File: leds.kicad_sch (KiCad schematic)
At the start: 6 parts, among them IC1 HT16K33

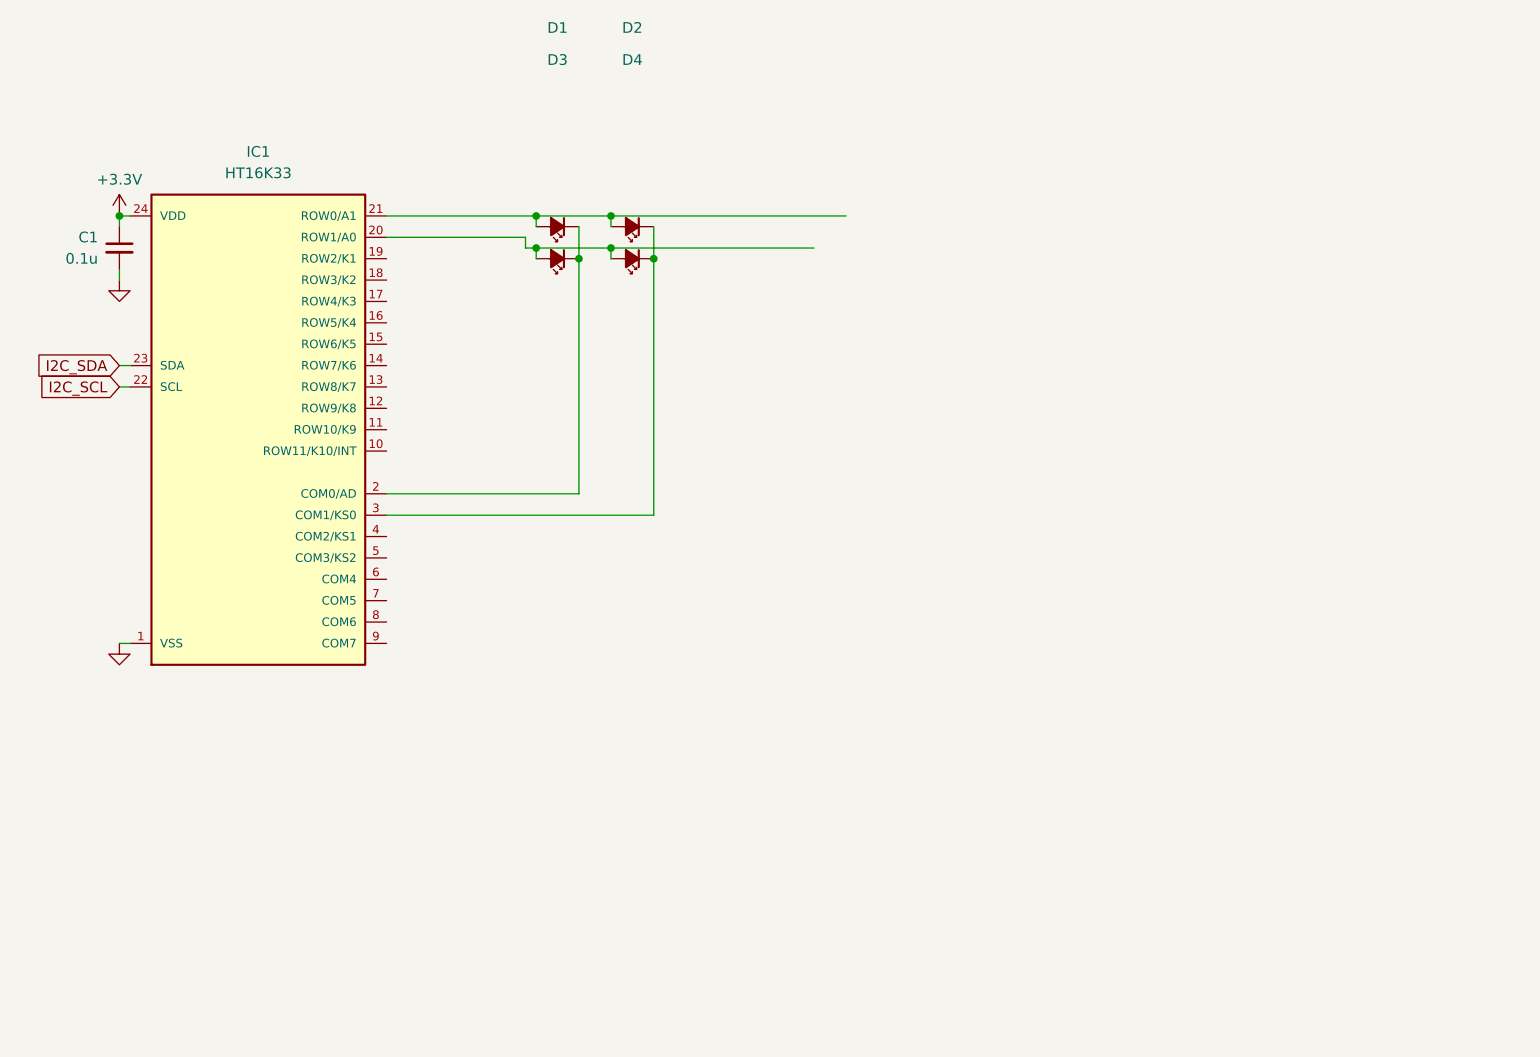
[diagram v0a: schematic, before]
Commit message: 251023
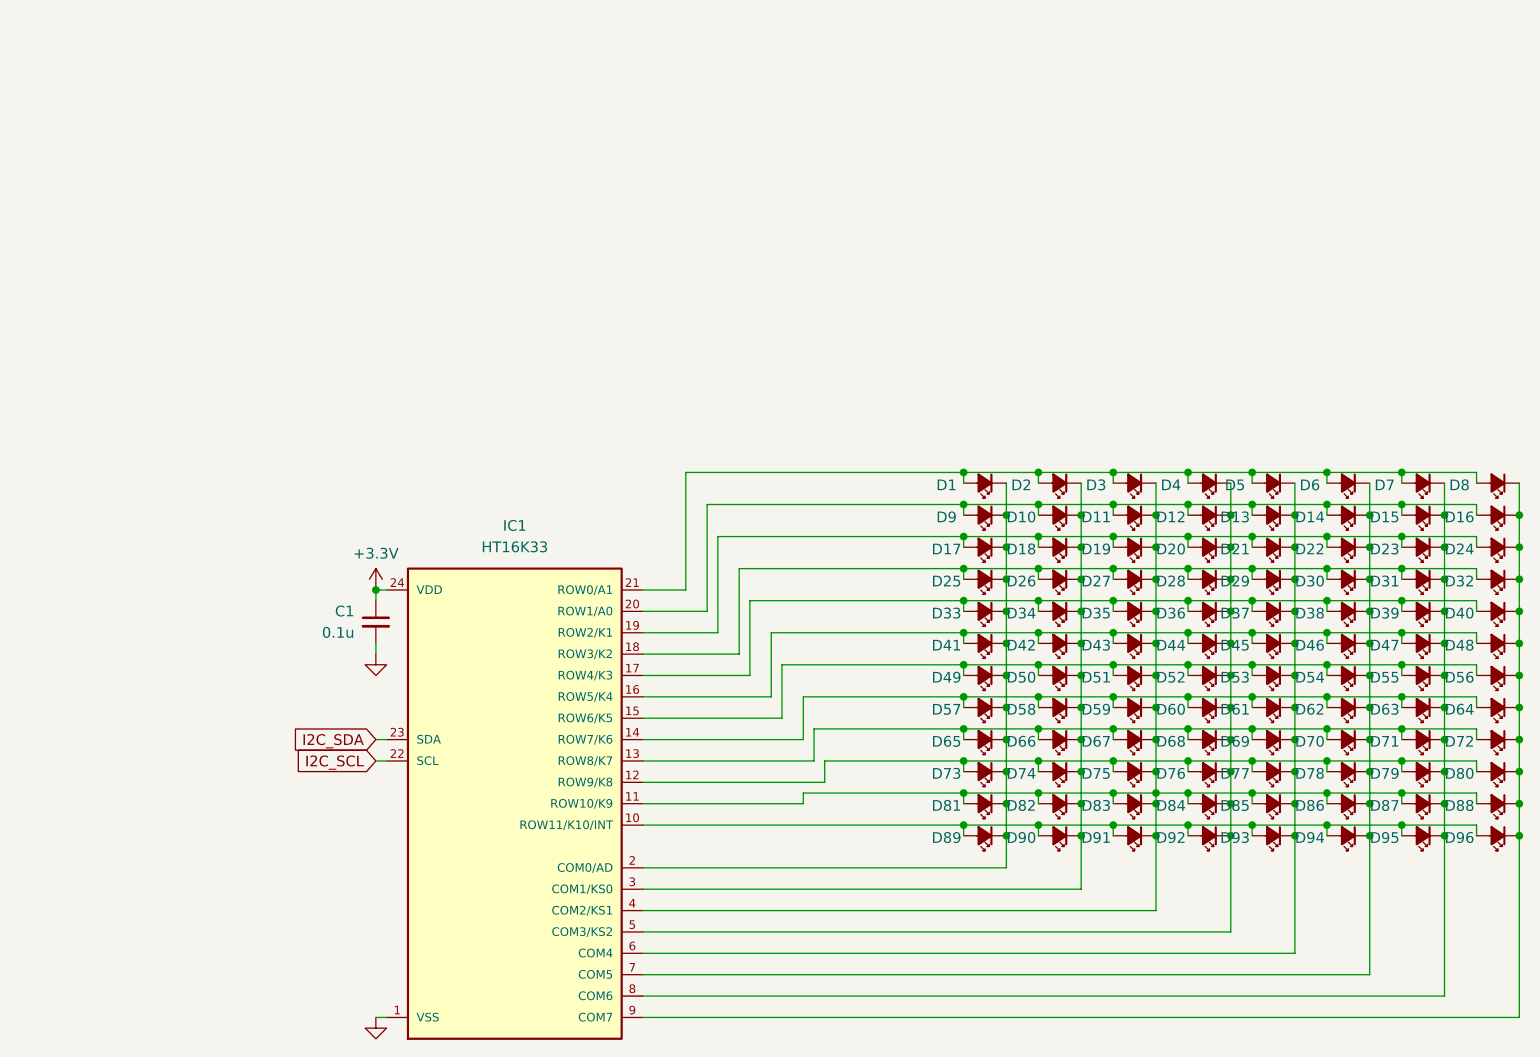
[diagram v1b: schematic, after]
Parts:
- added D11, D12, D13, D14, D15, D16, D17, D18, D19, D20, D21, D22, D23, D24, D25, D26, D27, D28, D29, D3, D30, D31, D32, D33, D34, D35, D36, D37, D38, D39, D4, D40, D41, D42, D43, D44, D45, D46, D47, D48, D49, D5, D50, D51, D52, D53, D54, D55, D56, D57, D58, D59, D6, D60, D61, D62, D63, D64, D65, D66, D67, D68, D69, D7, D70, D71, D72, D73, D74, D75, D76, D77, D78, D79, D8, D80, D81, D82, D83, D84, D85, D86, D87, D88, D89, D90, D91, D92, D93, D94, D95, D96: LED_Small_Filled, LED_SMD:LED_0603_1608Metric_Pad1.05x0.95mm_HandSolder, symbol Device:LED_Small_Filled
- renumbered D4 to D10, D3 to D9
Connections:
- net at D10.1 (K), D2.1 (K), IC1.3 (COM1/KS0): now also D18.1 (K), D26.1 (K), D34.1 (K), D42.1 (K), D50.1 (K), D58.1 (K), D66.1 (K), D74.1 (K), D82.1 (K), D90.1 (K)
- net at D10.2 (A), D9.2 (A), IC1.20 (ROW1/A0): now also D11.2 (A), D12.2 (A), D13.2 (A), D14.2 (A), D15.2 (A), D16.2 (A)
- net at D1.2 (A), D2.2 (A), IC1.21 (ROW0/A1): now also D3.2 (A), D4.2 (A), D5.2 (A), D6.2 (A), D7.2 (A), D8.2 (A)
- net at IC1.10 (ROW11/K10/INT): now also D89.2 (A), D90.2 (A), D91.2 (A), D92.2 (A), D93.2 (A), D94.2 (A), D95.2 (A), D96.2 (A)
- net at IC1.11 (ROW10/K9): now also IC1.4 (COM2/KS1), D11.1 (K), D19.1 (K), D27.1 (K), D3.1 (K), D35.1 (K), D43.1 (K), D51.1 (K), D59.1 (K), D67.1 (K), D75.1 (K), D81.2 (A), D82.2 (A), D83.1 (K), D83.2 (A), D84.2 (A), D85.2 (A), D86.2 (A), D87.2 (A), D88.2 (A), D91.1 (K)
- net at IC1.12 (ROW9/K8): now also D73.2 (A), D74.2 (A), D75.2 (A), D76.2 (A), D77.2 (A), D78.2 (A), D79.2 (A), D80.2 (A)
- net at IC1.13 (ROW8/K7): now also D65.2 (A), D66.2 (A), D67.2 (A), D68.2 (A), D69.2 (A), D70.2 (A), D71.2 (A), D72.2 (A)
- net at IC1.14 (ROW7/K6): now also D57.2 (A), D58.2 (A), D59.2 (A), D60.2 (A), D61.2 (A), D62.2 (A), D63.2 (A), D64.2 (A)
- net at IC1.15 (ROW6/K5): now also D49.2 (A), D50.2 (A), D51.2 (A), D52.2 (A), D53.2 (A), D54.2 (A), D55.2 (A), D56.2 (A)
- net at IC1.16 (ROW5/K4): now also D41.2 (A), D42.2 (A), D43.2 (A), D44.2 (A), D45.2 (A), D46.2 (A), D47.2 (A), D48.2 (A)
- net at IC1.17 (ROW4/K3): now also D33.2 (A), D34.2 (A), D35.2 (A), D36.2 (A), D37.2 (A), D38.2 (A), D39.2 (A), D40.2 (A)
- net at IC1.18 (ROW3/K2): now also D25.2 (A), D26.2 (A), D27.2 (A), D28.2 (A), D29.2 (A), D30.2 (A), D31.2 (A), D32.2 (A)
- net at IC1.19 (ROW2/K1): now also D17.2 (A), D18.2 (A), D19.2 (A), D20.2 (A), D21.2 (A), D22.2 (A), D23.2 (A), D24.2 (A)
- net at D1.1 (K), D9.1 (K), IC1.2 (COM0/AD): now also D17.1 (K), D25.1 (K), D33.1 (K), D41.1 (K), D49.1 (K), D57.1 (K), D65.1 (K), D73.1 (K), D81.1 (K), D89.1 (K)
- net at IC1.5 (COM3/KS2): now also D12.1 (K), D20.1 (K), D28.1 (K), D36.1 (K), D4.1 (K), D44.1 (K), D52.1 (K), D60.1 (K), D68.1 (K), D76.1 (K), D84.1 (K), D92.1 (K)
- net at IC1.6 (COM4): now also D13.1 (K), D21.1 (K), D29.1 (K), D37.1 (K), D45.1 (K), D5.1 (K), D53.1 (K), D61.1 (K), D69.1 (K), D77.1 (K), D85.1 (K), D93.1 (K)
- net at IC1.7 (COM5): now also D14.1 (K), D22.1 (K), D30.1 (K), D38.1 (K), D46.1 (K), D54.1 (K), D6.1 (K), D62.1 (K), D70.1 (K), D78.1 (K), D86.1 (K), D94.1 (K)
- net at IC1.8 (COM6): now also D15.1 (K), D23.1 (K), D31.1 (K), D39.1 (K), D47.1 (K), D55.1 (K), D63.1 (K), D7.1 (K), D71.1 (K), D79.1 (K), D87.1 (K), D95.1 (K)
- net at IC1.9 (COM7): now also D16.1 (K), D24.1 (K), D32.1 (K), D40.1 (K), D48.1 (K), D56.1 (K), D64.1 (K), D72.1 (K), D8.1 (K), D80.1 (K), D88.1 (K), D96.1 (K)
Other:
- moved on the sheet: C1, D1, D10, D2, D9, IC1
